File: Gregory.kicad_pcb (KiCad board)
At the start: 2 copper layers, 104.2 x 96.5 mm, 43 parts, among them J1 Conn_01x03_Pin, SW1 SW_Push, SW10 SW_Push, SW11 SW_Push, SW12 SW_Push, SW13 SW_Push, SW14 SW_Push, SW15 SW_Push, SW16 SW_Push, SW17 RotaryEncoder, SW2 SW_Push, SW3 SW_Push, SW4 SW_Push, SW5 SW_Push, SW6 SW_Push, SW7 SW_Push, SW8 SW_Push, SW9 SW_Push, U1 MOUDLE-SEEEDUINO-XIAO, U2 ER_OLEDM0.91_1x-I2C

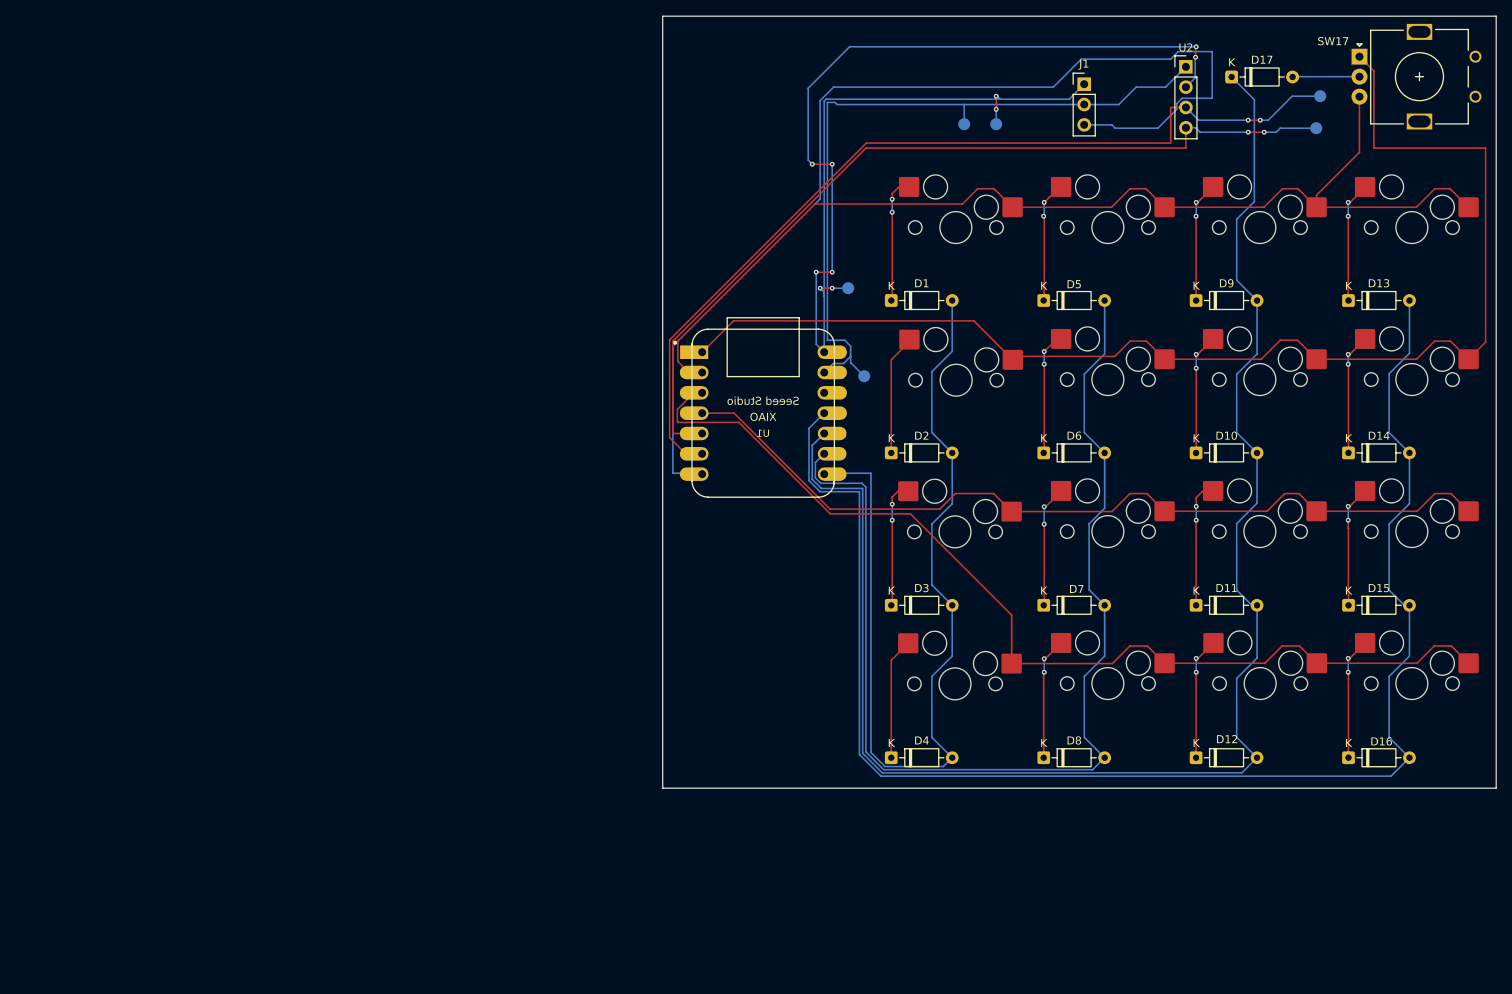
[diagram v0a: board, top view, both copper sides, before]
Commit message: Add files via upload
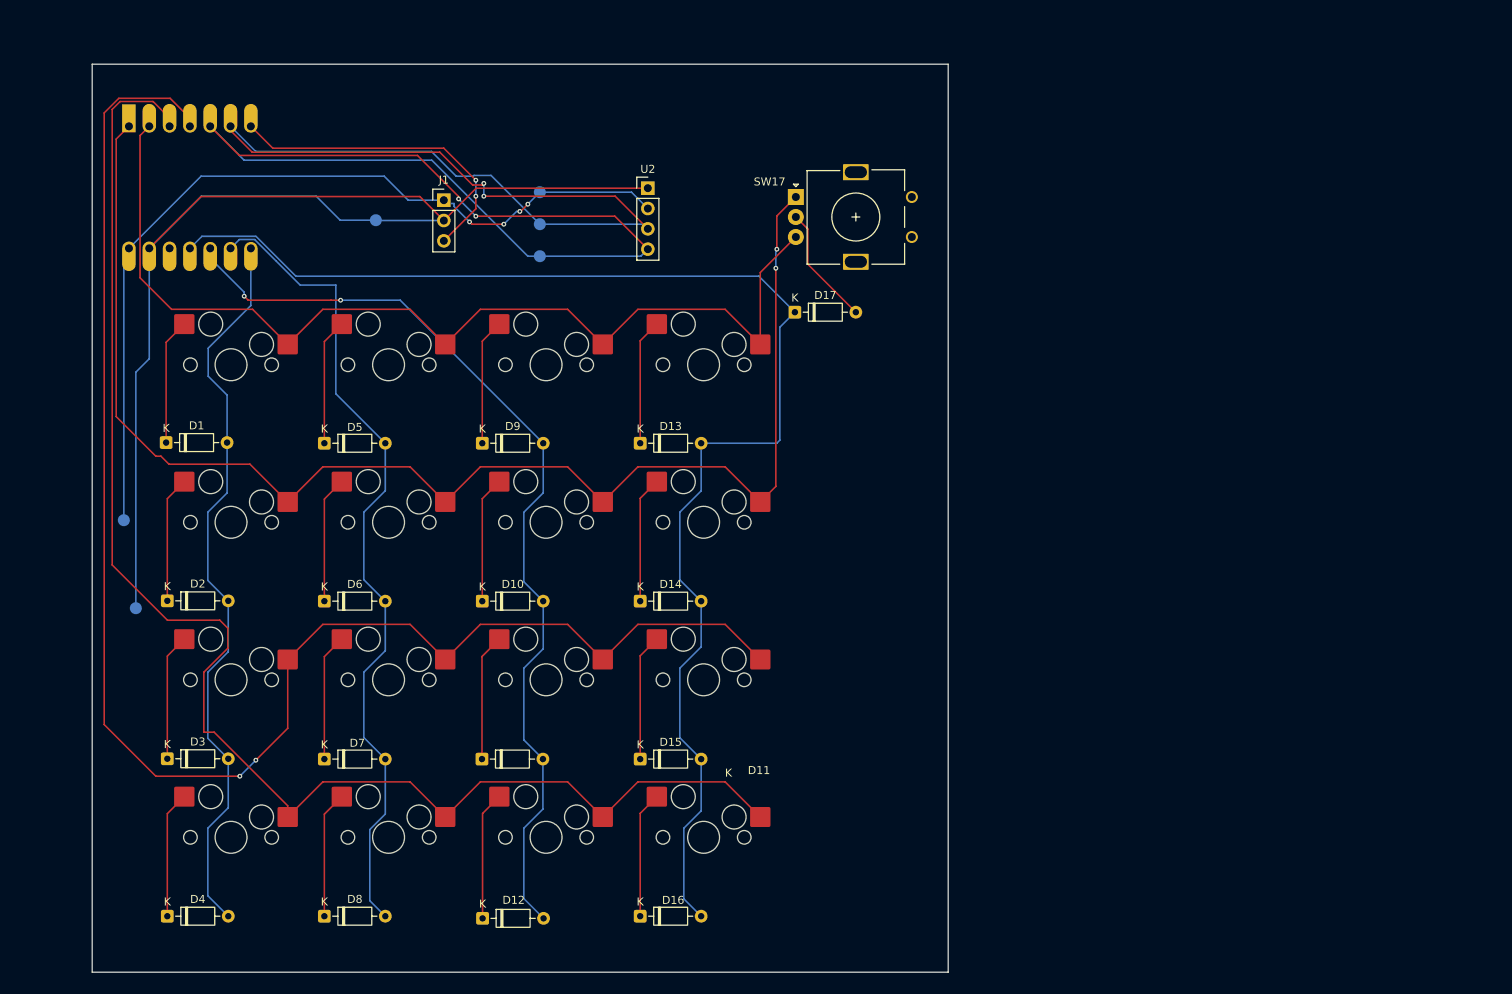
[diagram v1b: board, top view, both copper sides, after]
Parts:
- U1: moved to B.Cu
- moved TP4 98.8 mm to (115.5, 56.5)
- moved TP3 98.4 mm to (115.5, 60.5)
- moved TP1 95.6 mm to (65.0, 104.5)
- moved TP2 95.1 mm to (63.5, 93.5)
- moved D4 92.6 mm to (68.9, 143.0)
- moved D3 92.5 mm to (68.9, 123.3)
- moved SW4 92.5 mm to (76.9, 133.1)
- moved D1 92.4 mm to (68.7, 83.8)
- moved SW2 92.4 mm to (76.9, 93.8)
- moved SW3 92.4 mm to (76.9, 113.5)
- moved D2 92.4 mm to (68.9, 103.6)
- moved SW1 92.2 mm to (76.9, 74.1)
- moved D8 92.1 mm to (88.5, 143.0)
- moved D7 91.9 mm to (88.5, 123.4)
- moved SW8 91.9 mm to (96.5, 133.1)
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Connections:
- net GND renamed /GND
- D17 pad 1: /Row2 -> /Row3
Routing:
- net /DI: track 133.4 -> 40.1 mm, vias 0 -> 2
- net /Column3: track 108.0 -> 195.3 mm, vias 0 -> 2
- net /Row2: track 191.9 -> 118.1 mm, vias 0 -> 2
- net /GND: track 91.5 -> 154.4 mm
- net /5V: track 168.1 -> 108.6 mm, vias 10 -> 4
- net /Column2: track 125.9 -> 183.0 mm
- net /Row1: track 137.7 -> 103.5 mm
- net /Row0: track 115.0 -> 93.1 mm
- net /I2C_SDA: track 108.5 -> 123.0 mm
- net /Column0: track 158.6 -> 172.7 mm, vias 0 -> 2
- net /Row3: track 182.6 -> 172.3 mm
- net /Column1: track 135.6 -> 126.6 mm
- net Net-(D17-A): track 8.38 -> 15.0 mm
- net /I2C_SCL: track 115.0 -> 115.9 mm
- net Net-(D12-K): track 15.4 -> 16.1 mm, vias 2 -> 0
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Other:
- board size 104.2 x 96.5 mm -> 107 x 113.5 mm

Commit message: Add files via upload
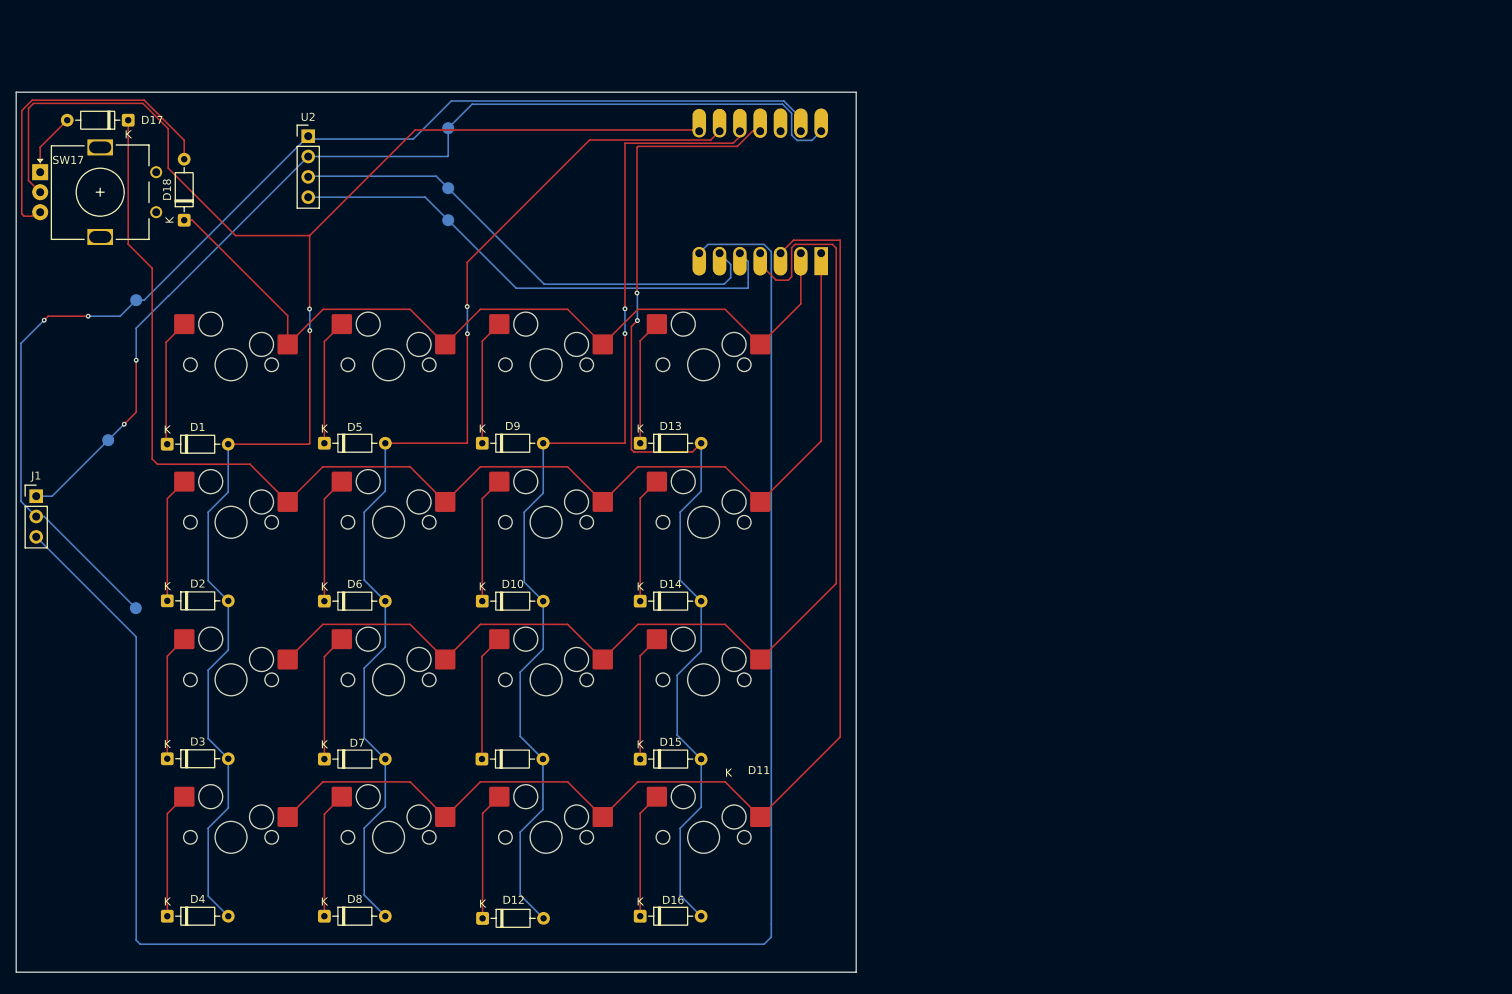
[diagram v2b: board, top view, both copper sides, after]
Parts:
- added D18: 1N4148, Diode_THT:D_DO-35_SOD27_P7.62mm_Horizontal, F.Cu at (71.0, 56.0)
- moved SW17 94.5 mm to (53.0, 50.0)
- moved D17 86.7 mm to (64.0, 43.5), turned to 180 degrees
- moved U1 71.3 mm to (143.0, 52.5), turned to 90 degrees
- moved J1 63.0 mm to (52.5, 90.5)
- moved U2 42.9 mm to (86.5, 45.5)
- moved TP6 31.6 mm to (65.0, 66.0)
- moved TP5 14.0 mm to (104.0, 44.5)
- moved TP3 12.3 mm to (104.0, 56.0)
- moved TP4 12.3 mm to (104.0, 52.0)
- moved TP2 10.2 mm to (61.5, 83.5)
- moved D1 0.24 mm to (68.9, 84.0)
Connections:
- D17 pad 1: /Row3 -> /Column0
- SW17 pad A: /Column0 -> Net-(D17-A)
- SW17 pad B: /Column1 -> Net-(D18-A)
- SW17 pad C: Net-(D17-A) -> /Row0
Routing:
- net /DI: track 40.1 -> 231.6 mm, vias 2 -> 0
- net /Row0: track 93.1 -> 212.0 mm, vias 0 -> 2
- net /I2C_SDA: track 123.0 -> 65.6 mm, vias 2 -> 0
- net /Column3: track 195.3 -> 141.2 mm, vias 2 -> 0
- net /I2C_SCL: track 115.9 -> 62.4 mm, vias 2 -> 0
- net /Row3: track 172.3 -> 129.6 mm, vias 0 -> 2
- net Net-(D18-A): track 0.00 -> 40.8 mm
- net /Row1: track 103.5 -> 136.8 mm, vias 0 -> 2
- net /Column2: track 183.0 -> 154.4 mm
- net /5V: track 108.6 -> 131.1 mm, vias 4 -> 2
- net /Column1: track 126.6 -> 105.0 mm
- net /Row2: track 118.1 -> 129.2 mm
- net Net-(D17-A): track 15.0 -> 7.90 mm
- net /Column0: track 172.7 -> 167.0 mm, vias 2 -> 0
- net /GND: track 154.4 -> 152.5 mm, vias 0 -> 2
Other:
- board size 107 x 113.5 mm -> 105 x 110 mm

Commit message: Add files via upload
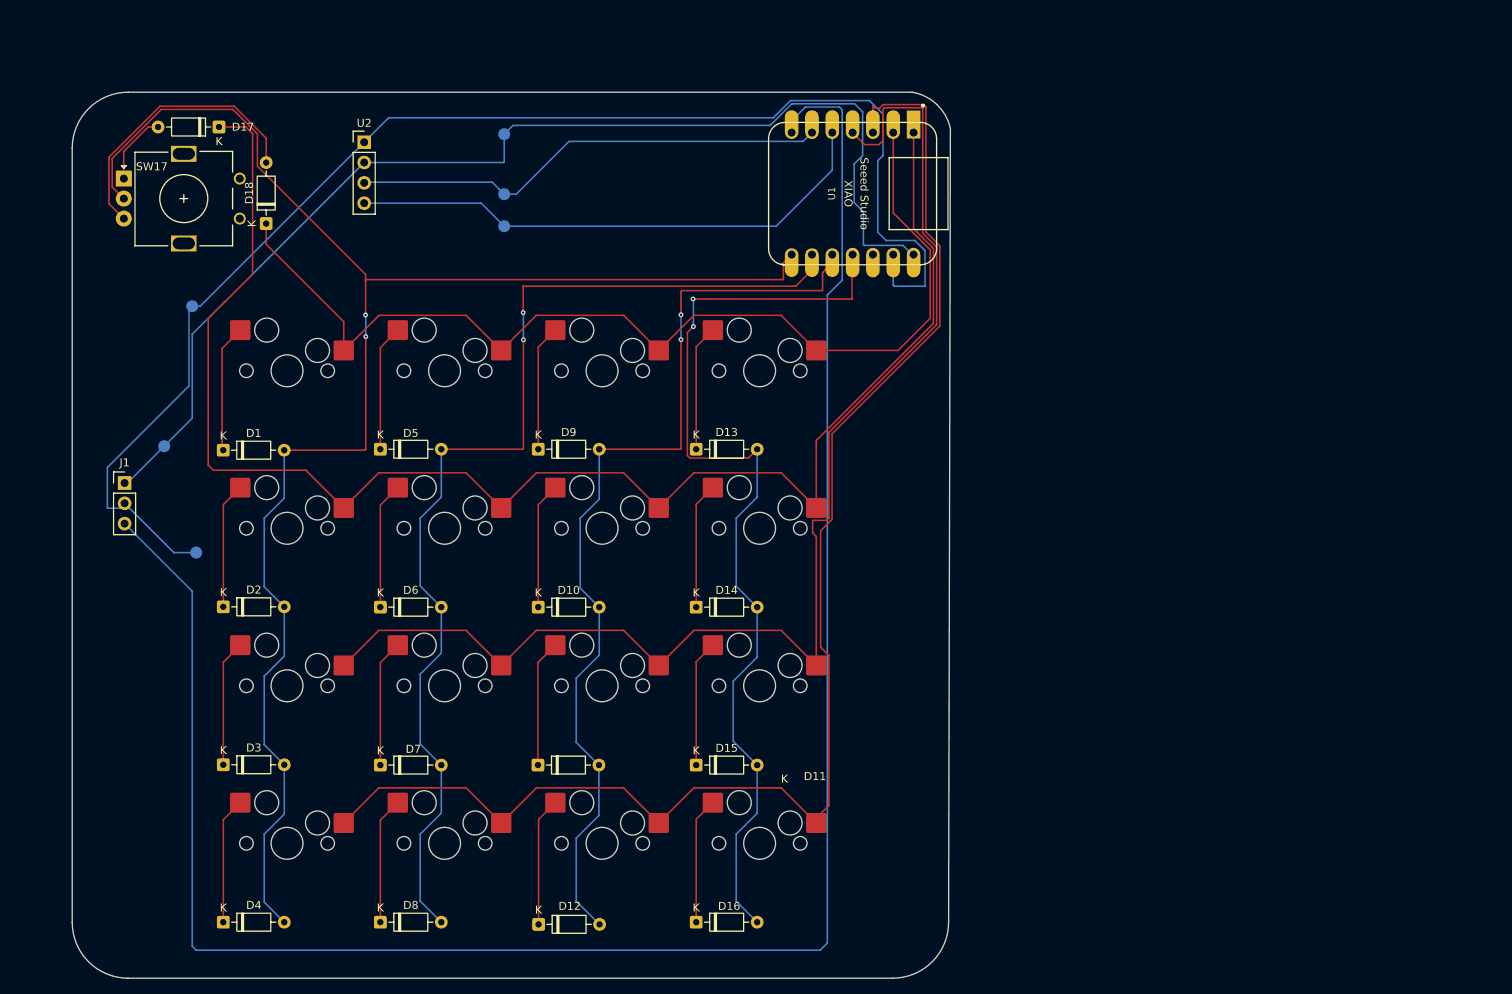
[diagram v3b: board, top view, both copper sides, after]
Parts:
- U1: moved to F.Cu
- moved U1 11.6 mm to (154.6, 52.7), turned to -90 degrees
- moved D17 11.4 mm to (75.3, 44.4)
- moved J1 11.2 mm to (63.5, 88.8)
- moved SW17 10.5 mm to (63.5, 50.8)
- moved D18 10.3 mm to (81.2, 56.4)
- moved TP1 10.3 mm to (72.5, 97.5)
- moved D1 7.04 mm to (75.9, 84.8)
- moved D10 7.04 mm to (115.3, 104.4)
- moved D11 7.04 mm to (115.2, 124.1)
- moved D12 7.04 mm to (115.3, 144.0)
- moved D13 7.04 mm to (135.0, 84.6)
- moved D14 7.04 mm to (135.0, 104.4)
- moved D15 7.04 mm to (135.0, 124.1)
- moved D16 7.04 mm to (135.0, 143.8)
- moved D2 7.04 mm to (75.9, 104.3)
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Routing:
- net /Column1: track 105.0 -> 130.9 mm
- net /Column0: track 167.0 -> 191.4 mm
- net /Column2: track 154.4 -> 178.3 mm
- net /GND: track 152.5 -> 175.9 mm, vias 2 -> 0
- net /Column3: track 141.2 -> 162.5 mm
- net /DI: track 231.6 -> 249.9 mm
- net /5V: track 131.1 -> 145.4 mm, vias 2 -> 0
- net /Row2: track 129.2 -> 118.7 mm
- net /Row3: track 129.6 -> 120.6 mm
- net /Row0: track 212.0 -> 204.2 mm
- net Net-(D18-A): track 40.8 -> 35.4 mm
- net /I2C_SDA: track 65.6 -> 67.3 mm
- net /Row1: track 136.8 -> 135.1 mm
- net Net-(D17-A): track 7.90 -> 8.94 mm
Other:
- board size 105 x 110 mm -> 109.8 x 110.8 mm
